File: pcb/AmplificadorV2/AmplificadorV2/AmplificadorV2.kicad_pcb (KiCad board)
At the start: 2 copper layers, 2 parts, among them U1 MHT2012N

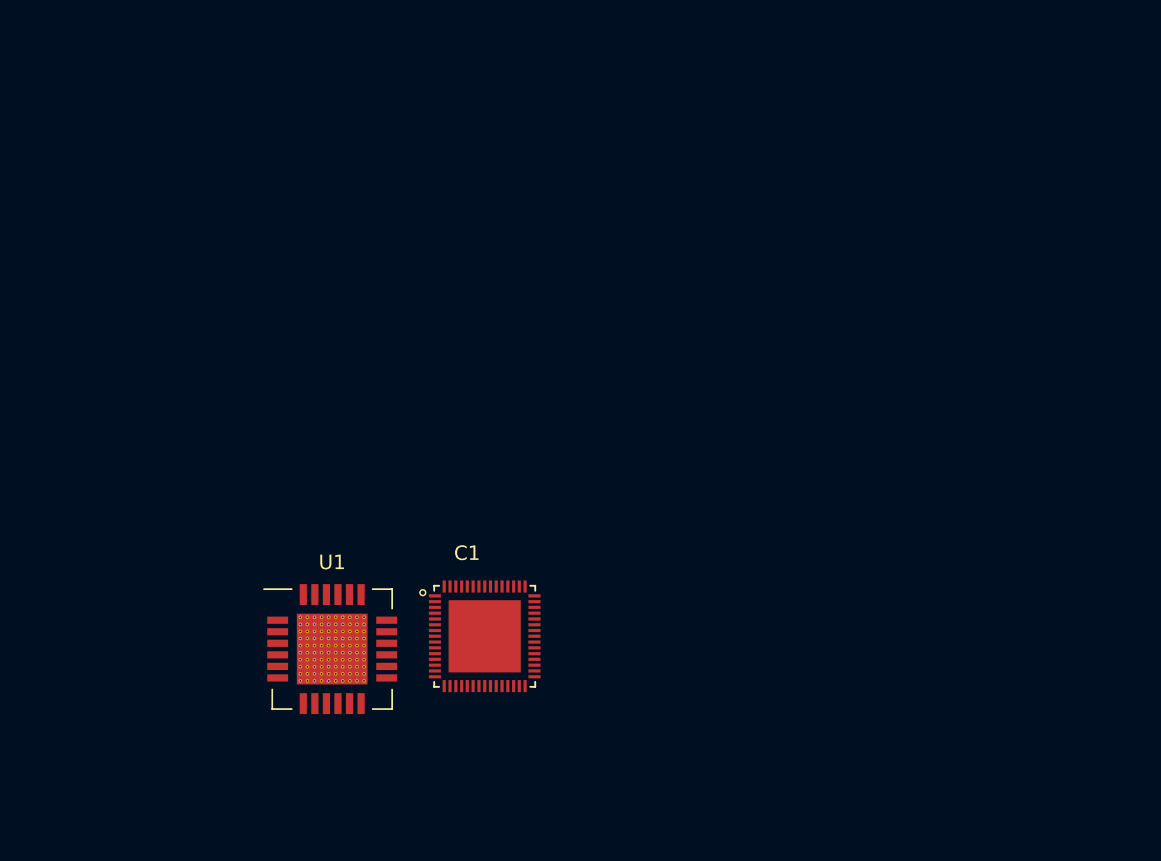
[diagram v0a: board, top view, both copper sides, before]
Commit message: ampli terminado
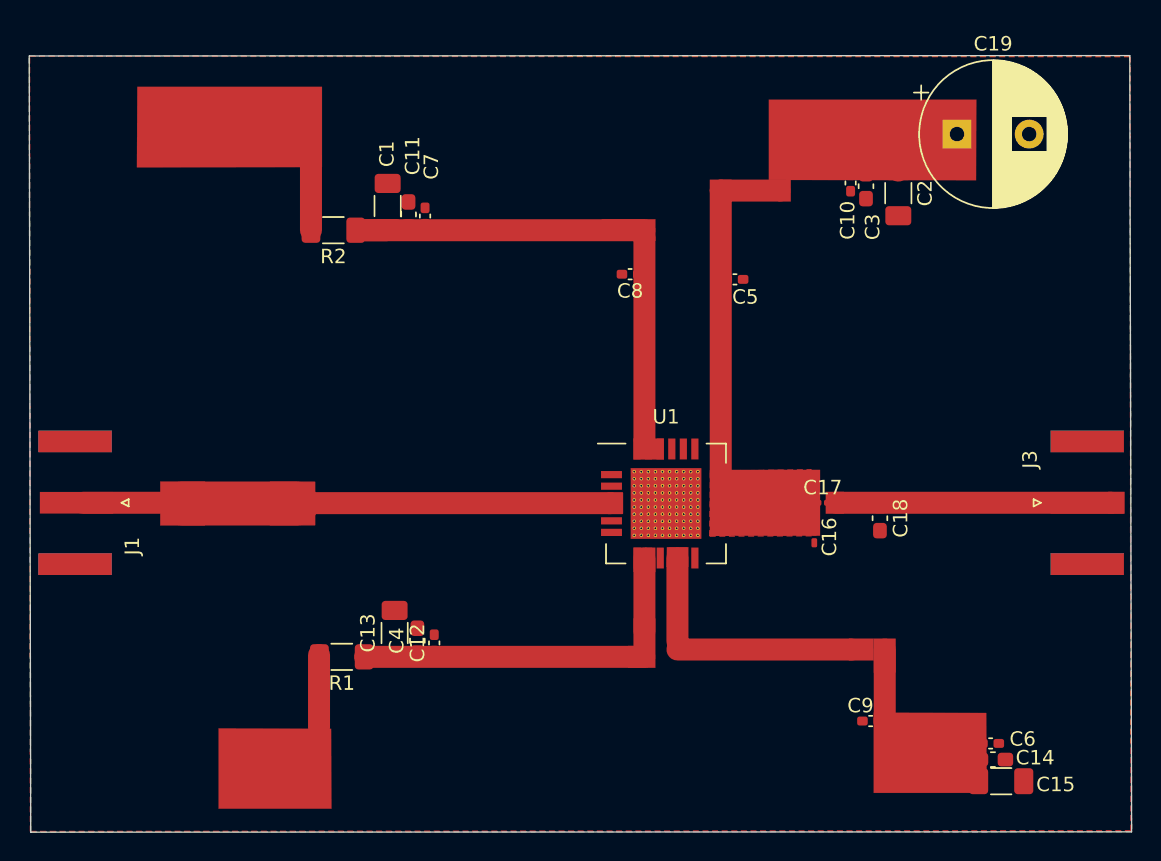
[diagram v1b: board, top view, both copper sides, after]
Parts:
- added C10: 5.6pF, Capacitor_SMD:C_0402_1005Metric_Pad0.74x0.62mm_HandSolder, F.Cu at (40.9, -27.2)
- added C11: 0.1uF, Capacitor_SMD:C_0603_1608Metric_Pad1.08x0.95mm_HandSolder, F.Cu at (10.3, -25.1)
- added C12: 5.6pF, Capacitor_SMD:C_0402_1005Metric_Pad0.74x0.62mm_HandSolder, F.Cu at (12.1, 4.60)
- added C13: 10uF, Capacitor_SMD:C_1206_3216Metric_Pad1.33x1.80mm_HandSolder, F.Cu at (9.35, 3.91)
- added C14: 0.1uF, Capacitor_SMD:C_0603_1608Metric_Pad1.08x0.95mm_HandSolder, F.Cu at (50.8, 12.7)
- added C15: 10uF, Capacitor_SMD:C_1206_3216Metric_Pad1.33x1.80mm_HandSolder, F.Cu at (51.3, 14.2)
- added C16: 1.6pF, Capacitor_SMD:C_0201_0603Metric_Pad0.64x0.40mm_HandSolder, F.Cu at (38.4, -2.74)
- added C17: 4.7pF, Capacitor_SMD:C_0201_0603Metric_Pad0.64x0.40mm_HandSolder, F.Cu at (39.0, -5.11)
- added C18: 0.5pF, Capacitor_SMD:C_0603_1608Metric_Pad1.08x0.95mm_HandSolder, F.Cu at (43.0, -4.04)
- added C19: 220uF, Capacitor_THT:CP_Radial_D10.0mm_P5.00mm, F.Cu at (48.3, -30.6)
- added C2: 10uF, Capacitor_SMD:C_1206_3216Metric_Pad1.33x1.80mm_HandSolder, F.Cu at (44.2, -26.5)
- added C3: 0.1uF, Capacitor_SMD:C_0603_1608Metric_Pad1.08x0.95mm_HandSolder, F.Cu at (42.0, -27.0)
- added C4: 0.1uF, Capacitor_SMD:C_0603_1608Metric_Pad1.08x0.95mm_HandSolder, F.Cu at (10.9, 4.45)
- added C5: 5.6pF, Capacitor_SMD:C_0402_1005Metric_Pad0.74x0.62mm_HandSolder, F.Cu at (32.9, -20.6)
- added C6: 5.6pF, Capacitor_SMD:C_0402_1005Metric_Pad0.74x0.62mm_HandSolder, F.Cu at (50.6, 11.6)
- added C7: 5.6pF, Capacitor_SMD:C_0402_1005Metric_Pad0.74x0.62mm_HandSolder, F.Cu at (11.5, -25.0)
- added C8: 5.6pF, Capacitor_SMD:C_0402_1005Metric_Pad0.74x0.62mm_HandSolder, F.Cu at (25.7, -20.9)
- added C9: 5.6pF, Capacitor_SMD:C_0402_1005Metric_Pad0.74x0.62mm_HandSolder, F.Cu at (42.3, 10.0)
- added J1: Conn_01x01_Female, Connector_Coaxial:SMA_Amphenol_132289_EdgeMount, F.Cu at (-12.8, -5.11)
- added J3: Conn_01x01_Female, Connector_Coaxial:SMA_Amphenol_132289_EdgeMount, F.Cu at (57.3, -5.11)
- added R1: 4.7K, Resistor_SMD:R_1206_3216Metric_Pad1.30x1.75mm_HandSolder, F.Cu at (5.69, 5.56)
- added R2: 4.7k, Resistor_SMD:R_1206_3216Metric_Pad1.30x1.75mm_HandSolder, F.Cu at (5.10, -24.0)
- C1: value C -> 10uF; footprint FootprintAmpli:QFN40P700X700X75-61N -> Capacitor_SMD:C_1206_3216Metric_Pad1.33x1.80mm_HandSolder
- moved C1 30.5 mm to (8.86, -25.7), turned to 90 degrees
- moved U1 25.2 mm to (28.1, -5.05)
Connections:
- net Net-(J1-Pad1) renamed Rfin
- U1 pad 10: Net-(C12-Pad1) -> outAmpli
- U1 pad 11: Net-(U1-Pad11) -> outAmpli
- U1 pad 14: Net-(U1-Pad14) -> (no net)
- U1 pad 15: Net-(C10-Pad1) -> (no net)
- U1 pad 16: Net-(C10-Pad1) -> (no net)
- U1 pad 17: Net-(U1-Pad17) -> (no net)
- U1 pad 18: Net-(U1-Pad18) -> (no net)
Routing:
- net (no net): track 0.00 -> 45.8 mm
- net Rfin: track 0.00 -> 34.6 mm
- net Net-(U1-Pad23): track 0.00 -> 33.3 mm
- net Net-(C1-Pad1): track 0.00 -> 24.4 mm
- net outAmpli: track 0.00 -> 22.9 mm
- net Net-(C2-Pad1): track 0.00 -> 5.11 mm
- net Net-(J2-Pad1): track 0.00 -> 5.02 mm
- net Net-(R1-Pad2): track 0.00 -> 5.02 mm
- added copper zone on B.Cu, net GND
- added copper zone on F.Cu, net GND
- added copper zone on In1.Cu, net GND
- added copper zone on In2.Cu, net GND
- added copper zone on F.Cu, net outAmpli
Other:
- board outline added: 76.3 x 53.8 mm
- copper layers 2 -> 4
- net class Default: trace_width 0.25 -> 1.524
- net class adaptador added: clearance 0.2, trace_width 3.048, via_dia 0.8, via_drill 0.4
